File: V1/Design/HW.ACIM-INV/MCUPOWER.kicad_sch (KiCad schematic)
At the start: 33 parts, among them J2 FAN, U10 LDO 5V±1%, U12 SMPS 12V±2%/0.8A, U13 LDO 3.3V±0.1%/20mA, U2 LDO 3V3±2%

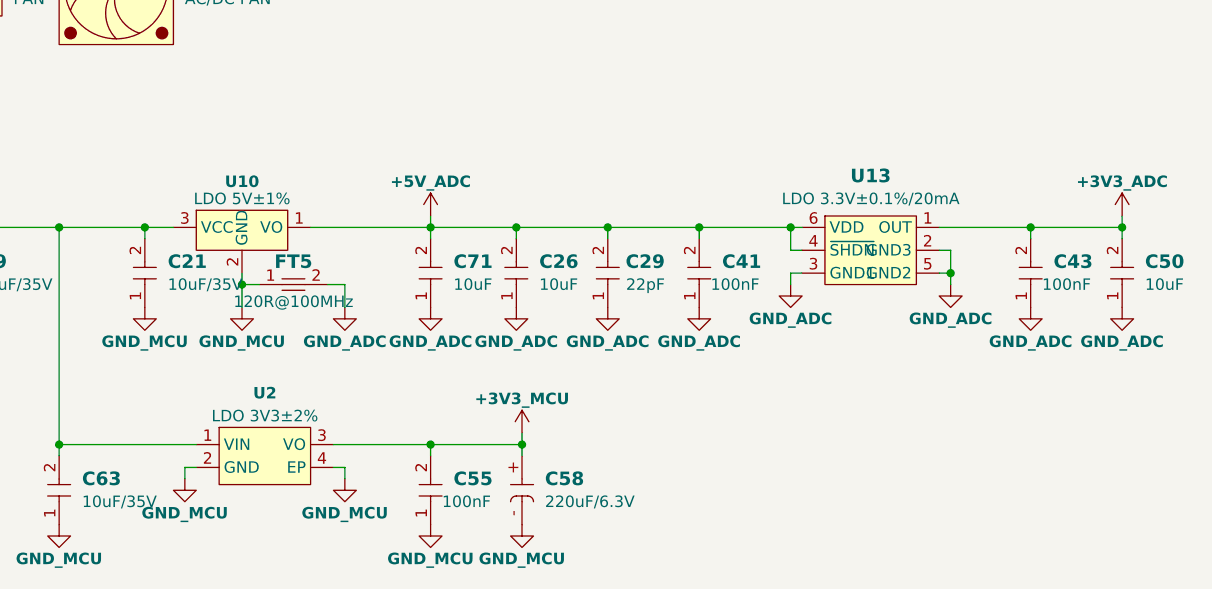
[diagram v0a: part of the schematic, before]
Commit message: V1 schematic update 15
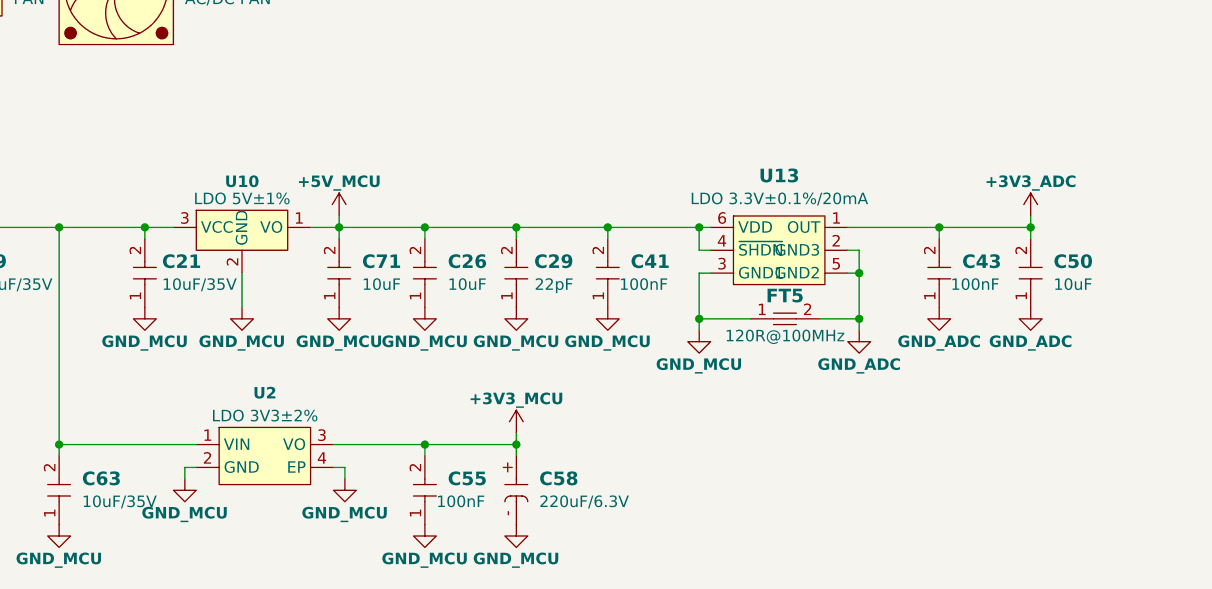
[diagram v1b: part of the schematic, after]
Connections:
- net GND_ADC: no longer C26.1, C29.1, C41.1, C71.1, U13.3 (GND1)
- net GND_MCU: now also C26.1, C29.1, C41.1, C71.1, U13.3 (GND1)
- net +5V_ADC renamed +5V_MCU
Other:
- company: TON DUC THANG UNIVERSITY -> (none)
- moved on the sheet: C26, C29, C41, C43, C50, C55, C58, C71, FT5, U13

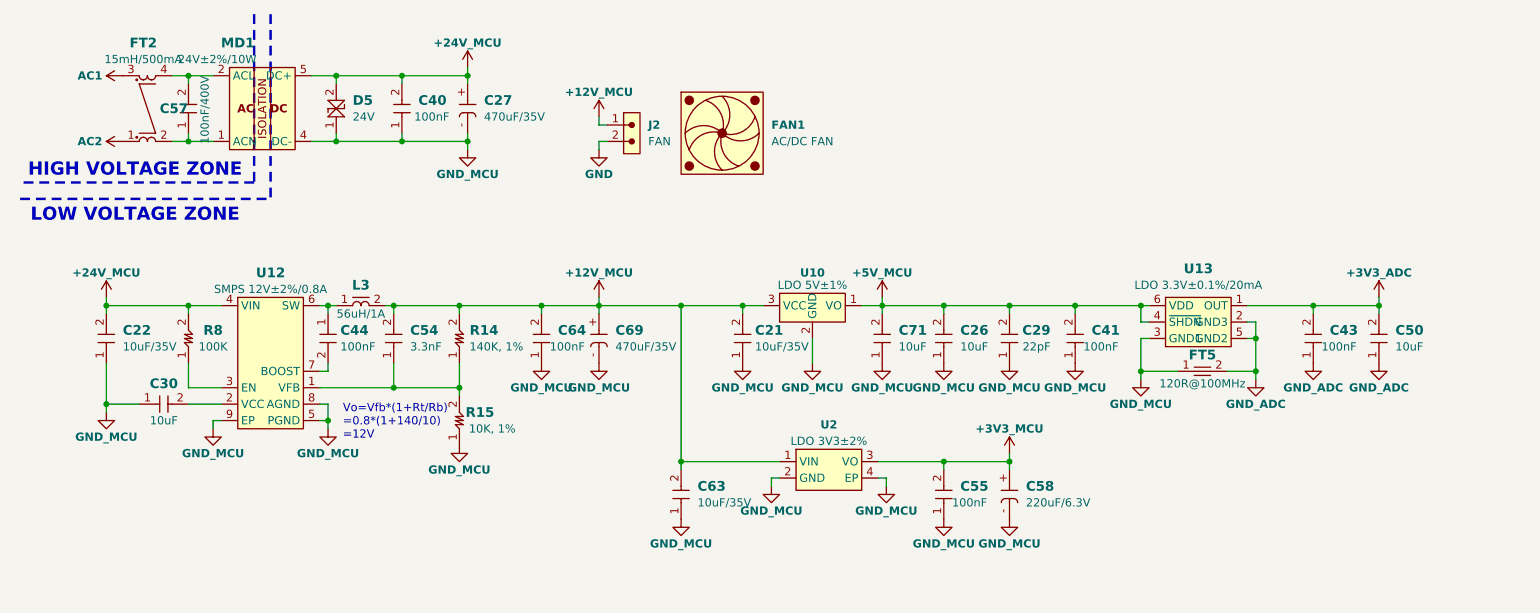
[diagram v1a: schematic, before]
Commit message: V1 schematic update 16
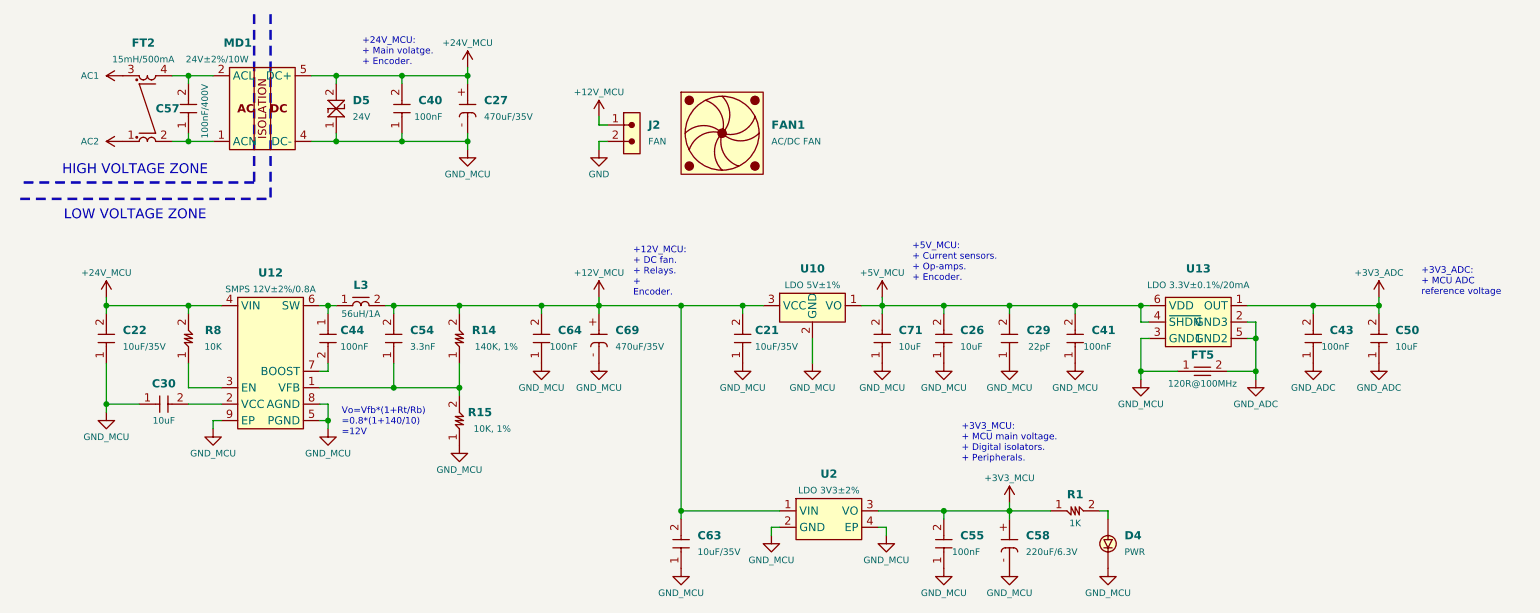
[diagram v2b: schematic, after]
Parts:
- added D4: PWR, SAMPI:LED0603, symbol SAMPI:WLED
- added R1: 1K, SAMPI:RES0603, symbol SAMPI:RES
- C21, C22, C63: footprint SAMPI:CAP0603 -> SAMPI:CAP1206; MFT Samsung -> (none); MNP CL10A106MQ8NNNC -> (none)
- C26, C50: Checked OK -> (none); Unit Price 0.079 -> (none)
- C29: Checked OK -> (none); Unit Price 0.012 -> (none)
- C41, C43: Checked OK -> (none); Unit Price 0.0146 -> (none)
- R8: value 100K -> 10K; MFT YAGEO -> (none); MNP RC0603FR-07100KL -> (none)
- U13: Checked OK -> (none); Unit Price 1 -> (none)
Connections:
- net +3V3_MCU: now also R1.1
- net GND_MCU: now also D4.K
- new net: D4.A, R1.2
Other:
- moved on the sheet: C55, C58, C63, U2
